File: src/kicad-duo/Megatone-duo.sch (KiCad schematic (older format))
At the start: 22 parts, among them P1 Classic, P2 Boost, P3 Gnd, SW1 LORLIN_2X6

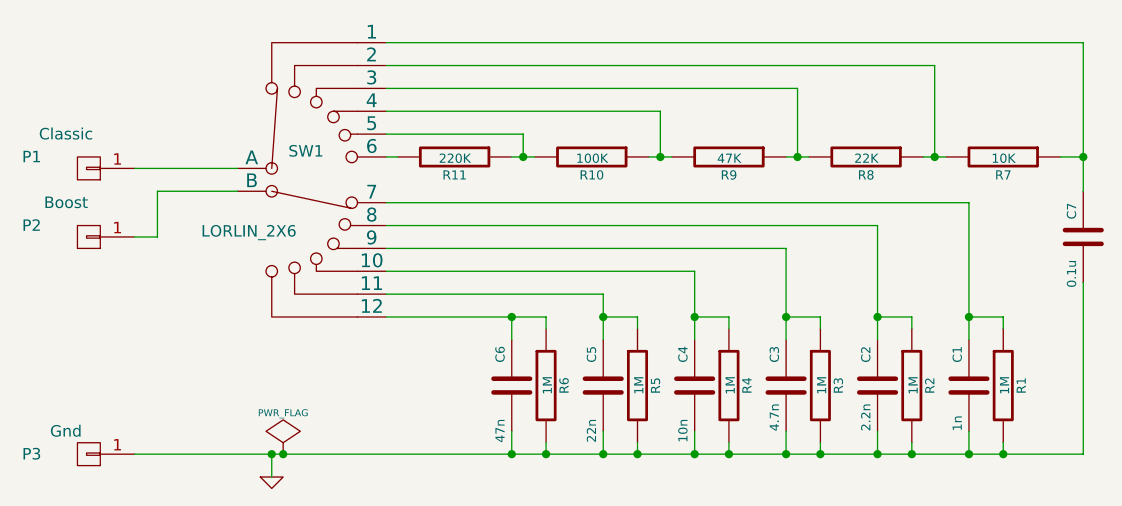
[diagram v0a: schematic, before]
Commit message: Revert "M. Duo: corrected wrong cap values on boost side"
This reverts commit b441f0806059993cadffced08bf4fcd550c3232b.
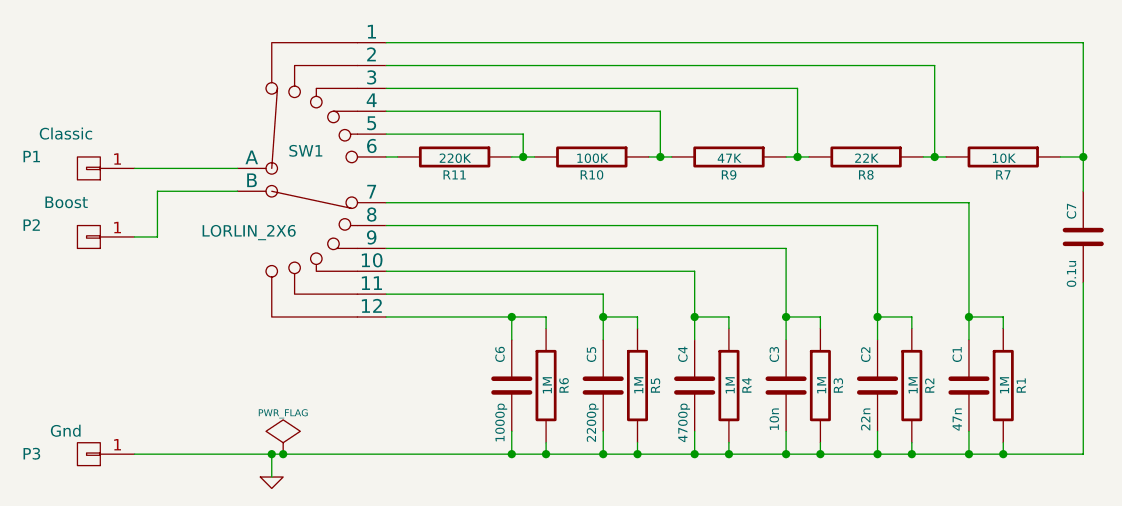
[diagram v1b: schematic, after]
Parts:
- C1: value 1n -> 47n
- C2: value 2.2n -> 22n
- C3: value 4.7n -> 10n
- C4: value 10n -> 4700p
- C5: value 22n -> 2200p
- C6: value 47n -> 1000p
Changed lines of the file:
@@
 P 8350 5750
 F 0 "C6" V 8300 5850 40  0000 L CNN
-F 1 "47n" V 8300 5500 40  0000 L CNN
+F 1 "1000p" V 8300 5500 40  0000 L CNN
 F 2 "libcms:SM0805" H 8388 5600 30  0001 C CNN
 F 3 "" H 8350 5750 60  0000 C CNN
@@
 P 8750 5750
 F 0 "C5" V 8700 5850 40  0000 L CNN
-F 1 "22n" V 8700 5500 40  0000 L CNN
+F 1 "2200p" V 8700 5500 40  0000 L CNN
 F 2 "libcms:SM0805" H 8788 5600 30  0001 C CNN
 F 3 "" H 8750 5750 60  0000 C CNN
@@
 P 9150 5750
 F 0 "C4" V 9100 5850 40  0000 L CNN
-F 1 "10n" V 9100 5500 40  0000 L CNN
+F 1 "4700p" V 9100 5500 40  0000 L CNN
 F 2 "libcms:SM0805" H 9188 5600 30  0001 C CNN
 F 3 "" H 9150 5750 60  0000 C CNN
@@
 P 9550 5750
 F 0 "C3" V 9500 5850 40  0000 L CNN
-F 1 "4.7n" V 9500 5550 40  0000 L CNN
+F 1 "10n" V 9500 5550 40  0000 L CNN
 F 2 "libcms:SM0805" H 9588 5600 30  0001 C CNN
 F 3 "" H 9550 5750 60  0000 C CNN
@@
 P 9950 5750
 F 0 "C2" V 9900 5850 40  0000 L CNN
-F 1 "2.2n" V 9900 5550 40  0000 L CNN
+F 1 "22n" V 9900 5550 40  0000 L CNN
 F 2 "libcms:SM0805" H 9988 5600 30  0001 C CNN
 F 3 "" H 9950 5750 60  0000 C CNN
@@
 P 10350 5750
 F 0 "C1" V 10300 5850 40  0000 L CNN
-F 1 "1n" V 10300 5550 40  0000 L CNN
+F 1 "47n" V 10300 5550 40  0000 L CNN
 F 2 "libcms:SM0805" H 10388 5600 30  0001 C CNN
 F 3 "" H 10350 5750 60  0000 C CNN

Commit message: M. Duo: corrected wrong cap values on boost side
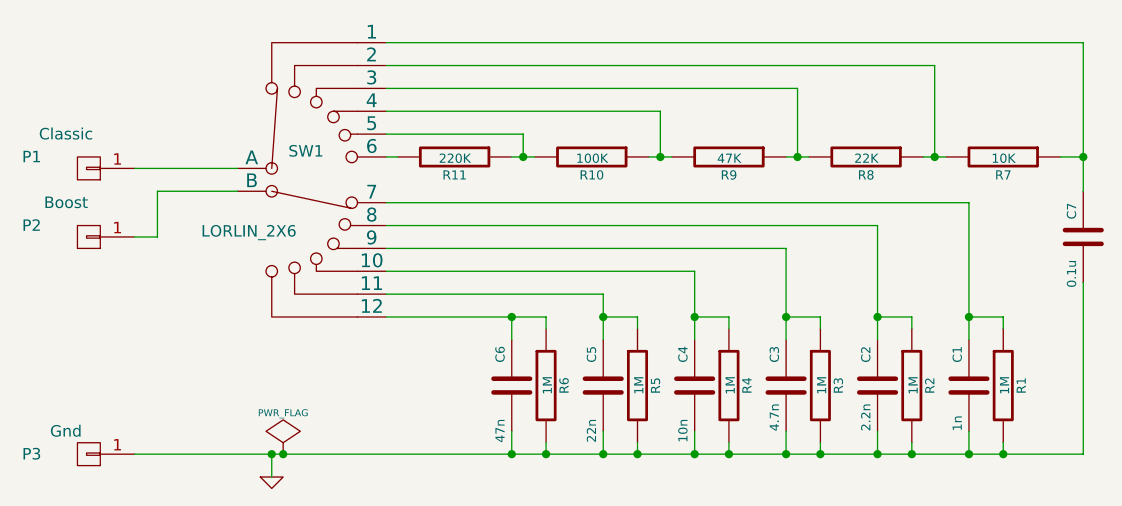
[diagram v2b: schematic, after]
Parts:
- C1: value 47n -> 1n
- C2: value 22n -> 2.2n
- C3: value 10n -> 4.7n
- C4: value 4700p -> 10n
- C5: value 2200p -> 22n
- C6: value 1000p -> 47n
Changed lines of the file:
@@
 P 8350 5750
 F 0 "C6" V 8300 5850 40  0000 L CNN
-F 1 "1000p" V 8300 5500 40  0000 L CNN
+F 1 "47n" V 8300 5500 40  0000 L CNN
 F 2 "libcms:SM0805" H 8388 5600 30  0001 C CNN
 F 3 "" H 8350 5750 60  0000 C CNN
@@
 P 8750 5750
 F 0 "C5" V 8700 5850 40  0000 L CNN
-F 1 "2200p" V 8700 5500 40  0000 L CNN
+F 1 "22n" V 8700 5500 40  0000 L CNN
 F 2 "libcms:SM0805" H 8788 5600 30  0001 C CNN
 F 3 "" H 8750 5750 60  0000 C CNN
@@
 P 9150 5750
 F 0 "C4" V 9100 5850 40  0000 L CNN
-F 1 "4700p" V 9100 5500 40  0000 L CNN
+F 1 "10n" V 9100 5500 40  0000 L CNN
 F 2 "libcms:SM0805" H 9188 5600 30  0001 C CNN
 F 3 "" H 9150 5750 60  0000 C CNN
@@
 P 9550 5750
 F 0 "C3" V 9500 5850 40  0000 L CNN
-F 1 "10n" V 9500 5550 40  0000 L CNN
+F 1 "4.7n" V 9500 5550 40  0000 L CNN
 F 2 "libcms:SM0805" H 9588 5600 30  0001 C CNN
 F 3 "" H 9550 5750 60  0000 C CNN
@@
 P 9950 5750
 F 0 "C2" V 9900 5850 40  0000 L CNN
-F 1 "22n" V 9900 5550 40  0000 L CNN
+F 1 "2.2n" V 9900 5550 40  0000 L CNN
 F 2 "libcms:SM0805" H 9988 5600 30  0001 C CNN
 F 3 "" H 9950 5750 60  0000 C CNN
@@
 P 10350 5750
 F 0 "C1" V 10300 5850 40  0000 L CNN
-F 1 "47n" V 10300 5550 40  0000 L CNN
+F 1 "1n" V 10300 5550 40  0000 L CNN
 F 2 "libcms:SM0805" H 10388 5600 30  0001 C CNN
 F 3 "" H 10350 5750 60  0000 C CNN
